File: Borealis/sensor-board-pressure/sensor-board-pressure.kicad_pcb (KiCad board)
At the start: 2 copper layers, 23.6 x 23.5 mm, 8 parts, among them U1 MAGNETIC POGO CONN., U2 MAGNETIC POGO CONN.

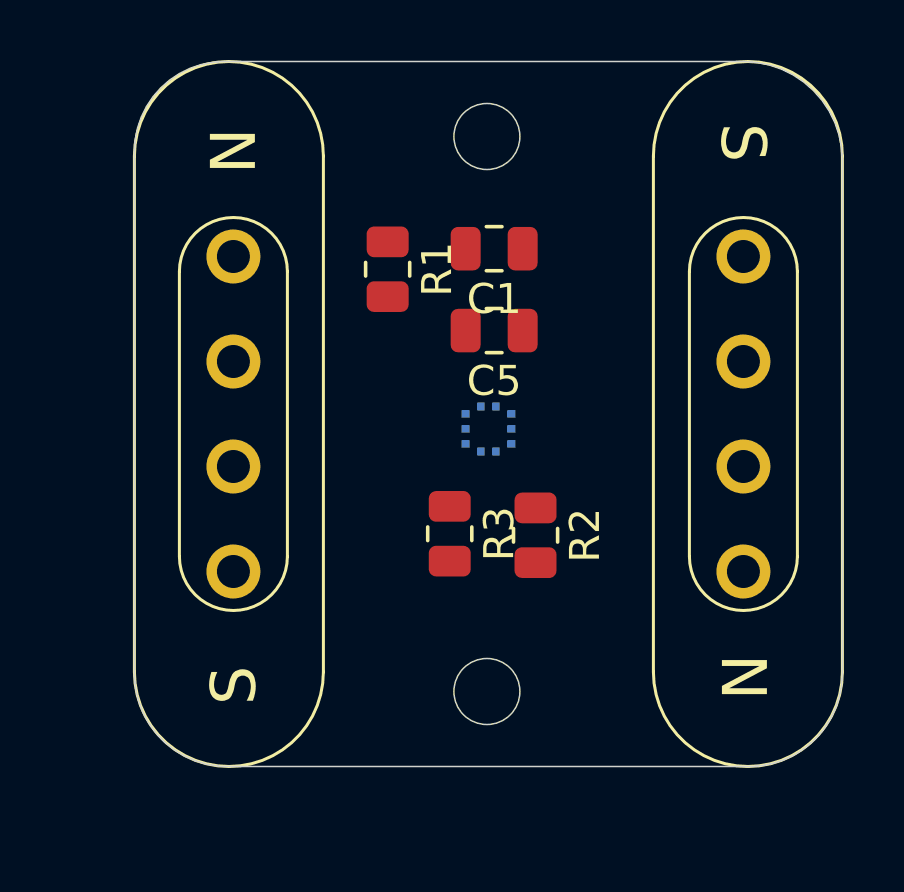
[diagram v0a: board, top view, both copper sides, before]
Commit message: Worked on boards
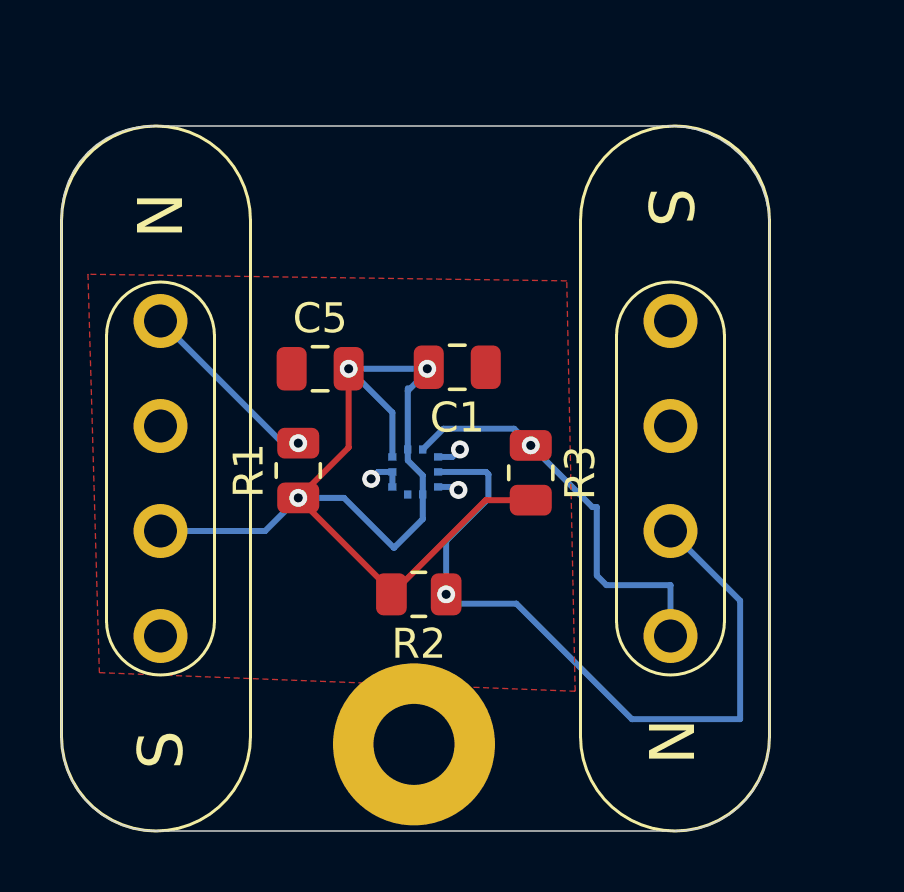
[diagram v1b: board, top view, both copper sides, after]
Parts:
- added H1: MountingHole, MountingHole:MountingHole_2.7mm_M2.5_Pad, F.Cu at (99.3, 74.8)
- moved R1 7.34 mm to (95.4, 65.6), turned to 90 degrees
- moved C5 5.94 mm to (96.1, 62.2), turned to 0 degrees
- moved R2 4.36 mm to (99.4, 69.8), turned to 180 degrees
- moved C1 4.14 mm to (100.7, 62.2)
- moved R3 3.38 mm to (103.2, 65.7)
- moved U1 3.24 mm to (107.8, 65.9)
- moved U2 3.24 mm to (90.8, 65.9)
- moved BMP390 2.83 mm to (99.3, 65.7), turned to 180 degrees
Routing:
- net +3.3V: track 0.07 -> 37.5 mm, vias 0 -> 3
- net /SDA: track 0.00 -> 25.1 mm, vias 0 -> 1
- net /SCL: track 0.00 -> 13.7 mm, vias 0 -> 1
- net /ID: track 0.00 -> 6.50 mm, vias 0 -> 1
- net GND: track 0.00 -> 2.85 mm, vias 0 -> 3
- added copper zone on F.Cu, net GND
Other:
- outline, holes or cut-outs redrawn
- board text added: "Borealis Pressure Sensor"
